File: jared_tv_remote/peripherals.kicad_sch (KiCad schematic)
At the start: 24 parts, among them Q1 Q_NPN, SW1 Power, SW10 Back, SW11 Home, SW12 Source, SW13 C1, SW14 C2, SW15 Learn, SW2 Up, SW3 Mute, SW4 Left, SW5 Select, SW6 Right, SW7 Vol-, SW8 Down, SW9 Vol+, U1 IRM-H638T, U4 E6QYDD1204-IRA940NM

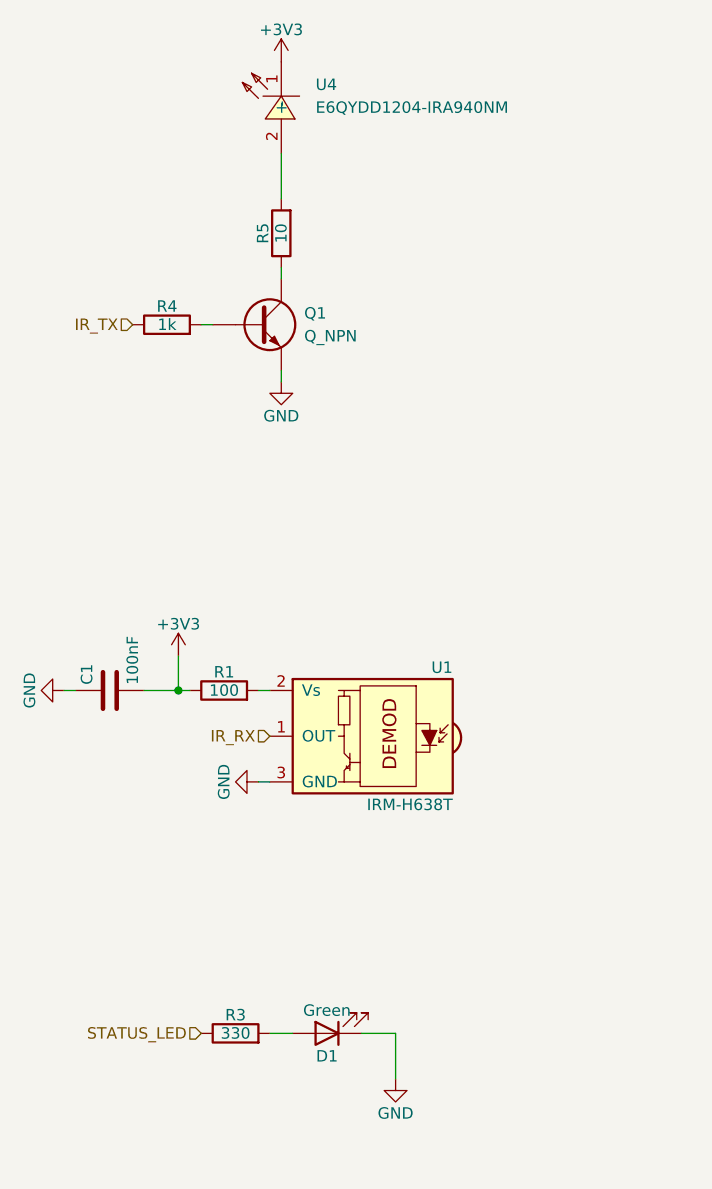
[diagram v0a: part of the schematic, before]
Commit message: new boards
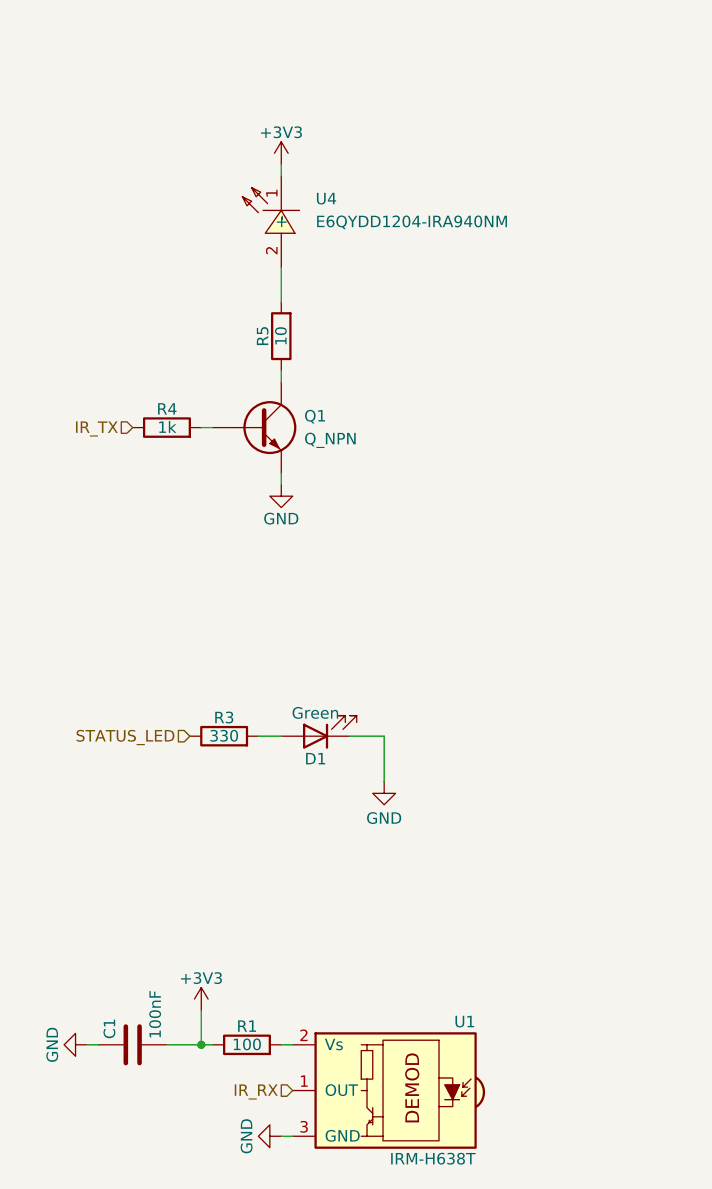
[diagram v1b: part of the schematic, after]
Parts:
- SW1, SW10, SW11, SW12, SW13, SW14, SW15, SW2, SW3, SW4, SW5, SW6, SW7, SW8, SW9: footprint Button_Switch_SMD:SW_SPST_B3U-1000P -> Button_Switch_SMD:SW_SPST_B3SL-1002P
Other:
- moved on the sheet: C1, D1, Q1, R1, R3, R4, R5, U1, U4
